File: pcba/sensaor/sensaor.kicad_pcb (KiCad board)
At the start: 2 copper layers, 18 parts, among them J1 SAO, J12 Conn_01x09_Pin, J13 Conn_01x09_Pin, J2 WS2812, J3 Conn_01x09_Pin, J4 Conn_01x09_Pin, J5 Conn_01x09_Pin, J6 Programming, J7 Speed, J8 Shape, J9 CONF, U1 CH32V003AxMx

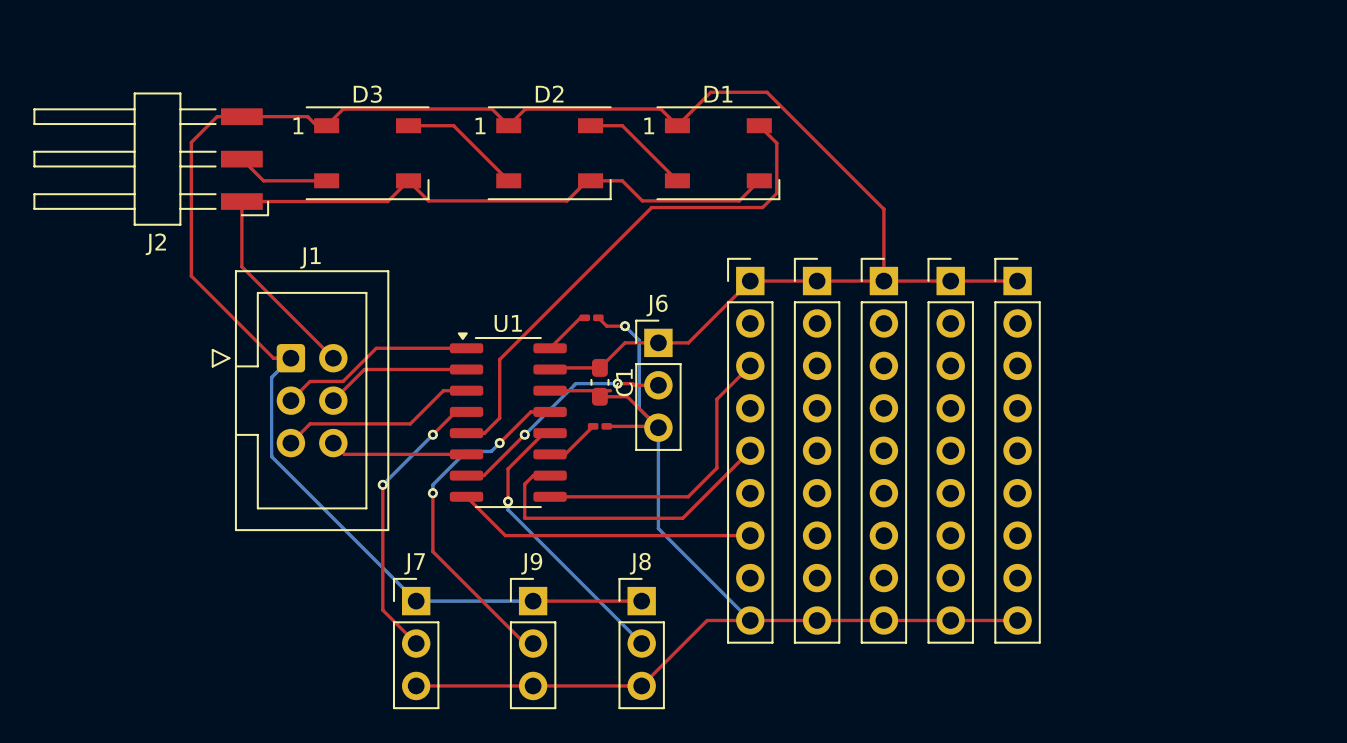
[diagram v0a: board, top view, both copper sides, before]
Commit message: Update PCB
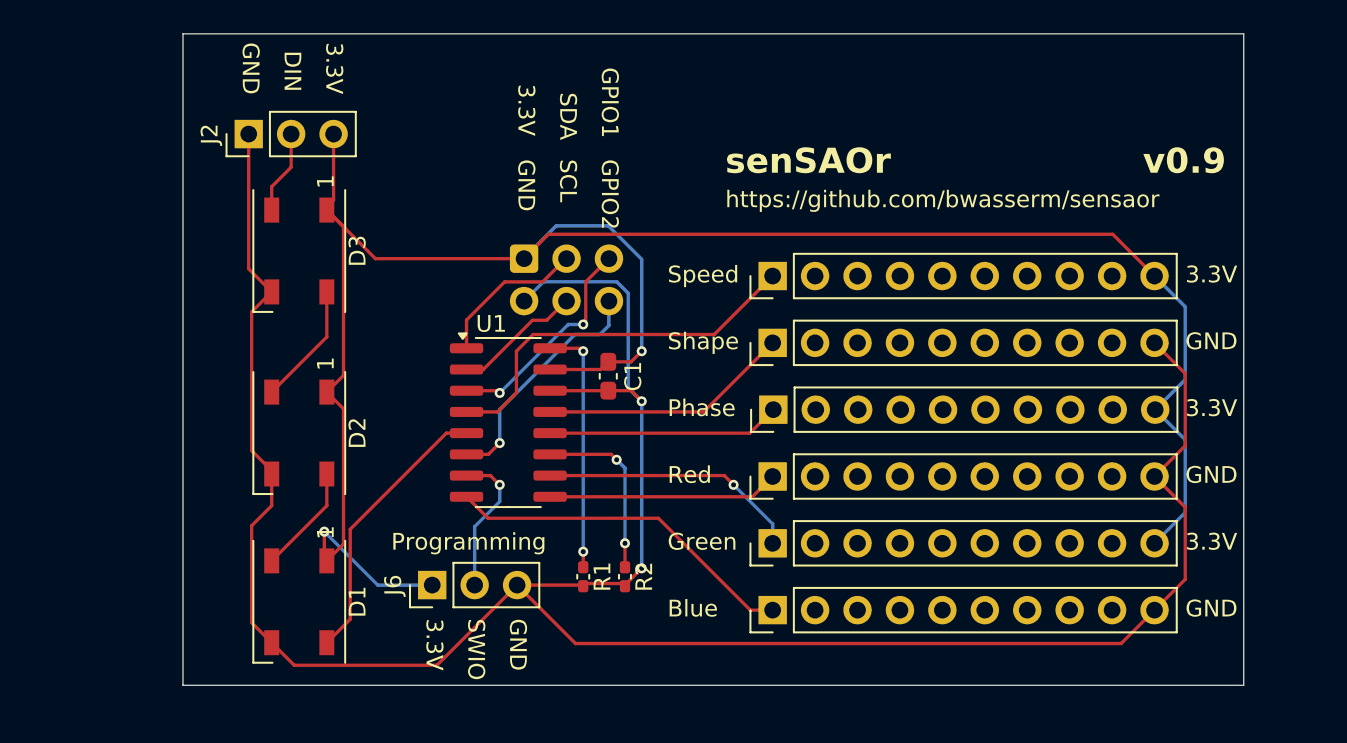
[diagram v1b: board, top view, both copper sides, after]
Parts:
- removed J12, J13: Conn_01x09_Pin, Connector_PinHeader_2.54mm:PinHeader_1x09_P2.54mm_Vertical
- J1: moved to B.Cu
- J2: footprint Connector_Harwin:Harwin_M20-89003xx_1x03_P2.54mm_Horizontal -> Connector_PinHeader_2.54mm:PinHeader_1x03_P2.54mm_Vertical
- J3, J4, J5: value Conn_01x09_Pin -> Conn_01x10_Pin; footprint Connector_PinHeader_2.54mm:PinHeader_1x09_P2.54mm_Vertical -> Connector_PinHeader_2.54mm:PinHeader_1x10_P2.54mm_Vertical
- J7: value Speed -> Conn_01x10_Pin; footprint Connector_PinHeader_2.54mm:PinHeader_1x03_P2.54mm_Vertical -> Connector_PinHeader_2.54mm:PinHeader_1x10_P2.54mm_Vertical
- J8: value Shape -> Conn_01x10_Pin; footprint Connector_PinHeader_2.54mm:PinHeader_1x03_P2.54mm_Vertical -> Connector_PinHeader_2.54mm:PinHeader_1x10_P2.54mm_Vertical
- J9: value CONF -> Conn_01x10_Pin; footprint Connector_PinHeader_2.54mm:PinHeader_1x03_P2.54mm_Vertical -> Connector_PinHeader_2.54mm:PinHeader_1x10_P2.54mm_Vertical
- R1, R2: footprint Resistor_SMD:R_0201_0603Metric_Pad0.64x0.40mm_HandSolder -> Capacitor_SMD:C_0402_1005Metric_Pad0.74x0.62mm_HandSolder
- moved D1 36.7 mm to (79.0, 79.5), turned to -90 degrees
- moved J7 22.6 mm to (107.3, 72.0), turned to 90 degrees
- moved D2 22.5 mm to (79.0, 69.4), turned to -90 degrees
- moved J6 19.8 mm to (87.0, 78.5), turned to 90 degrees
- moved R1 15.5 mm to (96.0, 78.0), turned to -90 degrees
- moved J1 15.2 mm to (92.5, 59.0), turned to -90 degrees
- moved J9 14.4 mm to (107.3, 80.0), turned to 90 degrees
- moved J5 10.2 mm to (107.4, 68.0), turned to 90 degrees
- moved R2 9.12 mm to (98.5, 78.0), turned to -90 degrees
- moved J8 8.57 mm to (107.3, 76.0), turned to 90 degrees
- moved D3 7.14 mm to (79.0, 58.5), turned to -90 degrees
- moved J2 6.12 mm to (76.0, 51.5), turned to 90 degrees
- moved J4 4.56 mm to (107.3, 64.0), turned to 90 degrees
- moved J3 1.37 mm to (107.3, 60.0), turned to 90 degrees
- moved C1 0.62 mm to (97.5, 66.0)
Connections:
- net /LED0 renamed /LED
- J3 pad 1: VCC -> /SPEED
- J3 pad 3: /AR -> unconnected-(J3-Pin_3-Pad3)
- J3 pad 5: /AG -> unconnected-(J3-Pin_5-Pad5)
- J3 pad 7: /AB -> unconnected-(J3-Pin_7-Pad7)
- J3 pad 9: GND -> unconnected-(J3-Pin_9-Pad9)
- J4 pad 1: VCC -> /SHAPE
- J4 pad 9: GND -> unconnected-(J4-Pin_9-Pad9)
- J5 pad 1: VCC -> /PHASE
- J5 pad 9: GND -> unconnected-(J5-Pin_9-Pad9)
- J7 pad 1: VCC -> /AR
- J7 pad 2: /SPEED -> unconnected-(J7-Pin_2-Pad2)
- J7 pad 3: GND -> unconnected-(J7-Pin_3-Pad3)
- J8 pad 1: VCC -> /AG
- J8 pad 2: /SHAPE -> unconnected-(J8-Pin_2-Pad2)
- J8 pad 3: GND -> unconnected-(J8-Pin_3-Pad3)
- J9 pad 1: VCC -> /AB
- J9 pad 2: /CONF -> unconnected-(J9-Pin_2-Pad2)
- J9 pad 3: GND -> unconnected-(J9-Pin_3-Pad3)
- U1 pad 12: /SHAPE -> /PHASE
- U1 pad 13: /CONF -> /SHAPE
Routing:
- net GND: track 116.3 -> 147.7 mm, vias 1 -> 2
- net /CONF: track 21.5 -> 0.00 mm, vias 2 -> 0
- net /LED: track 31.1 -> 16.7 mm
- net /PHASE: track 0.00 -> 13.9 mm
- net /ID0: track 2.83 -> 15.1 mm, vias 0 -> 2
- net /ID1: track 3.27 -> 10.9 mm, vias 0 -> 2
- net /SPEED: track 17.2 -> 23.2 mm, vias 2 -> 0
- net /GPIO2: track 8.50 -> 14.4 mm, vias 0 -> 1
- net /SWIO: track 13.8 -> 8.84 mm, vias 2 -> 1
- net /AR: track 17.6 -> 13.8 mm
- net /AG: track 18.9 -> 15.7 mm, vias 0 -> 1
- net /AB: track 17.9 -> 21.1 mm
- net /SDA: track 11.8 -> 9.16 mm
- net /SHAPE: track 17.2 -> 15.0 mm, vias 1 -> 0
- net VCC: track 130.2 -> 128.4 mm, vias 0 -> 2
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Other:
- board outline added: 63.5 x 39 mm
- board text added: "3.3V"
- board text added: "Blue"
- board text added: "DIN"
- board text added: "GND"
- board text added: "GPIO1"
- board text added: "GPIO2"
- board text added: "Green"
- board text added: "Phase"
- board text added: "Programming"
- board text added: "Red"
- board text added: "SCL"
- board text added: "SDA"
- board text added: "SWIO"
- board text added: "Shape"
- board text added: "Speed"
- board text added: "https://github.com/bwasserm/sensaor"
- board text added: "senSAOr"
- board text added: "v0.9"
